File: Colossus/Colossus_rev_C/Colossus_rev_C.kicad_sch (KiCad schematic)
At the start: 27 parts, among them J1 SWD, J2 Right Header, J3 Left Header, U1 STM32H523HEY6TR, U3 LD56100DPU33R, Y1 25MHz

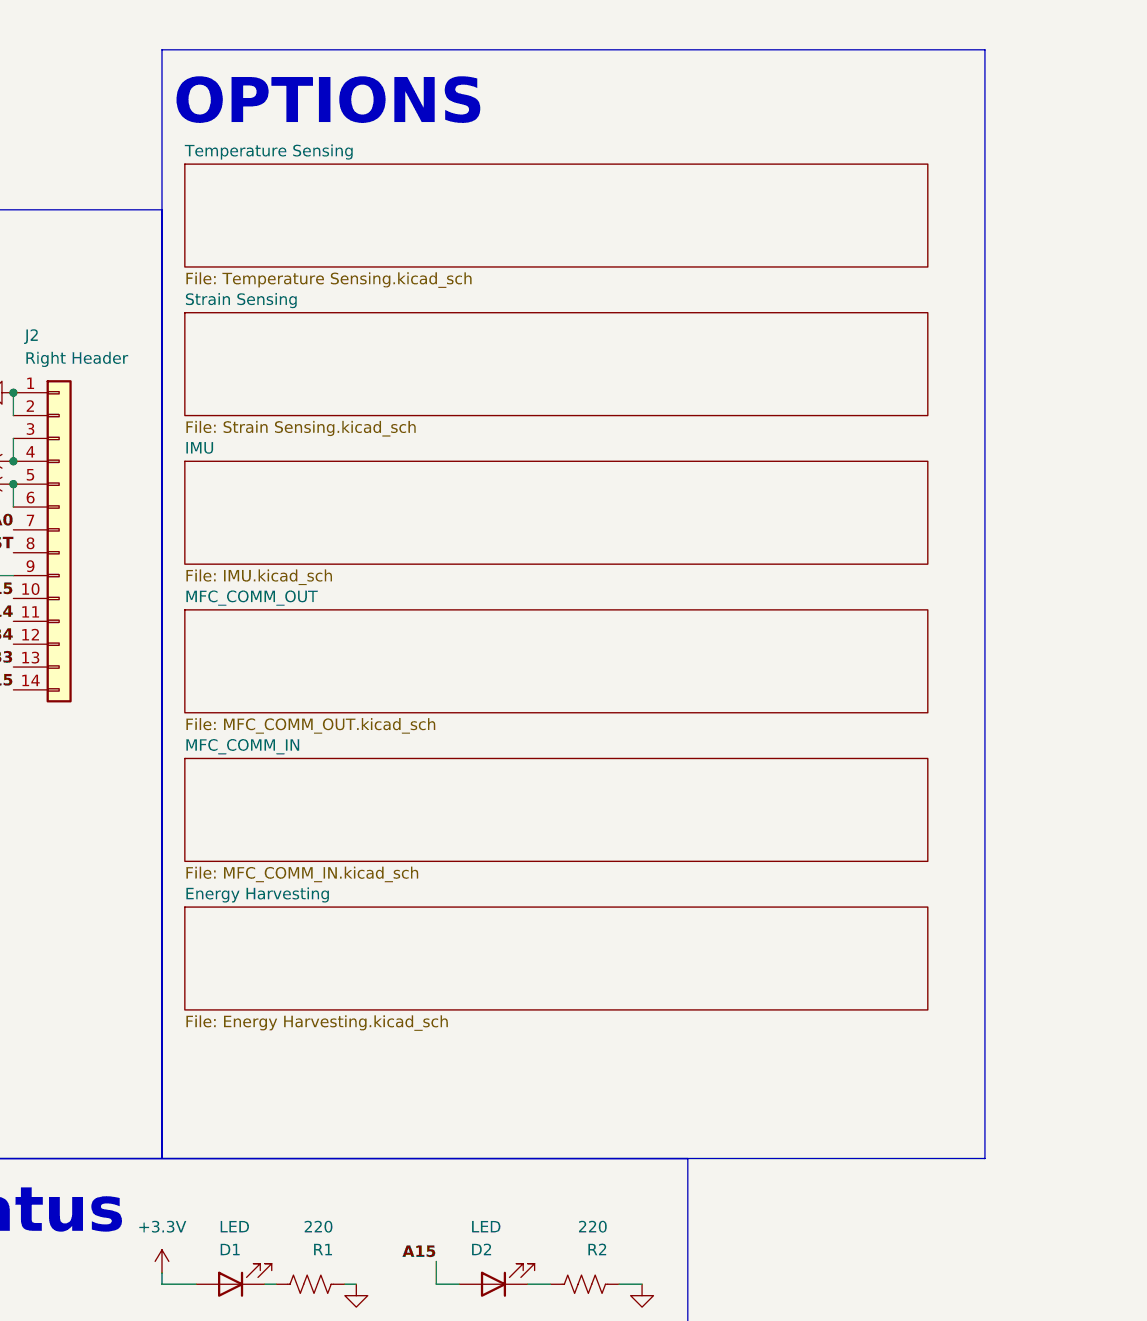
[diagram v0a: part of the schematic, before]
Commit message: pushing for desktop
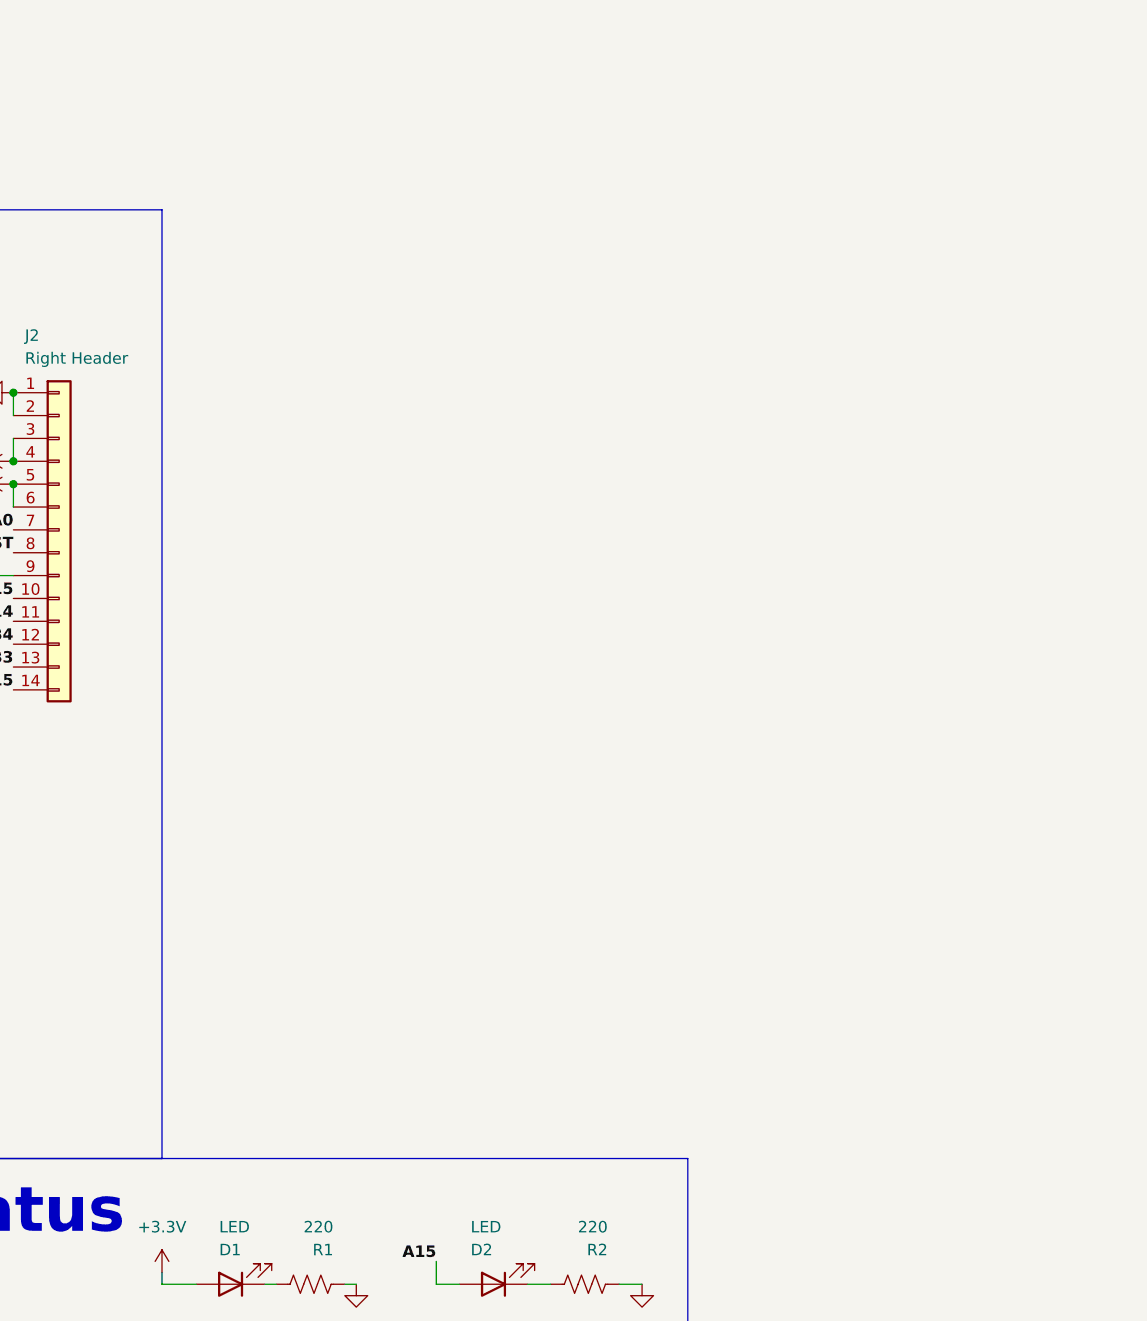
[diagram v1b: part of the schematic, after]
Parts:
- L1: footprint Inductor_SMD:L_APV_ANR252010 -> Inductor_SMD:L_0201_0603Metric
- U1: footprint Connector_PinHeader_1.27mm:PinHeader_1x14_P1.27mm_Horizontal -> Library:WLCSP39_STM
- U3: footprint Connector_PinHeader_1.27mm:PinHeader_1x14_P1.27mm_Vertical -> Library:DFN8_1P6X1P2_STM-M
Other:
- removed sheet Energy Harvesting
- removed sheet IMU
- removed sheet MFC_COMM_IN
- removed sheet MFC_COMM_OUT
- removed sheet Strain Sensing
- removed sheet Temperature Sensing
- note removed: "OPTIONS"
